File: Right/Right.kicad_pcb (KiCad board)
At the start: 2 copper layers, 106 parts, among them SW1 SW_PUSH, SW10 SW_PUSH, SW100 SW_Push_Dual_R, SW101 SW_Push_Dual_R, SW102 SW_Push_Dual_R, SW11 SW_PUSH, SW12 SW_PUSH, SW13 SW_PUSH, SW14 SW_PUSH, SW15 SW_PUSH, SW16 SW_PUSH, SW17 SW_PUSH, SW18 SW_PUSH, SW19 SW_PUSH, SW2 SW_PUSH, SW20 SW_PUSH, SW200 SW_SPDT, SW21 SW_PUSH, SW22 SW_PUSH, SW23 SW_PUSH, SW24 SW_PUSH, SW25 SW_PUSH, SW26 SW_PUSH, SW27 SW_PUSH, SW28 SW_PUSH, SW29 SW_PUSH, SW3 SW_PUSH, SW30 SW_PUSH, SW31 SW_PUSH, SW32 SW_PUSH, SW33 SW_PUSH, SW34 SW_PUSH, SW35 SW_PUSH, SW36 SW_PUSH, SW37 SW_PUSH, SW38 SW_PUSH, SW39 SW_PUSH, SW4 SW_PUSH, SW40 SW_PUSH, SW41 SW_PUSH, SW42 SW_PUSH, SW43 SW_PUSH, SW44 SW_PUSH, SW45 SW_PUSH, SW5 SW_PUSH, SW6 SW_PUSH, SW7 SW_PUSH, SW8 SW_PUSH, SW9 SW_PUSH, U1 CH25-2032LF, U2 CH25-2032LF

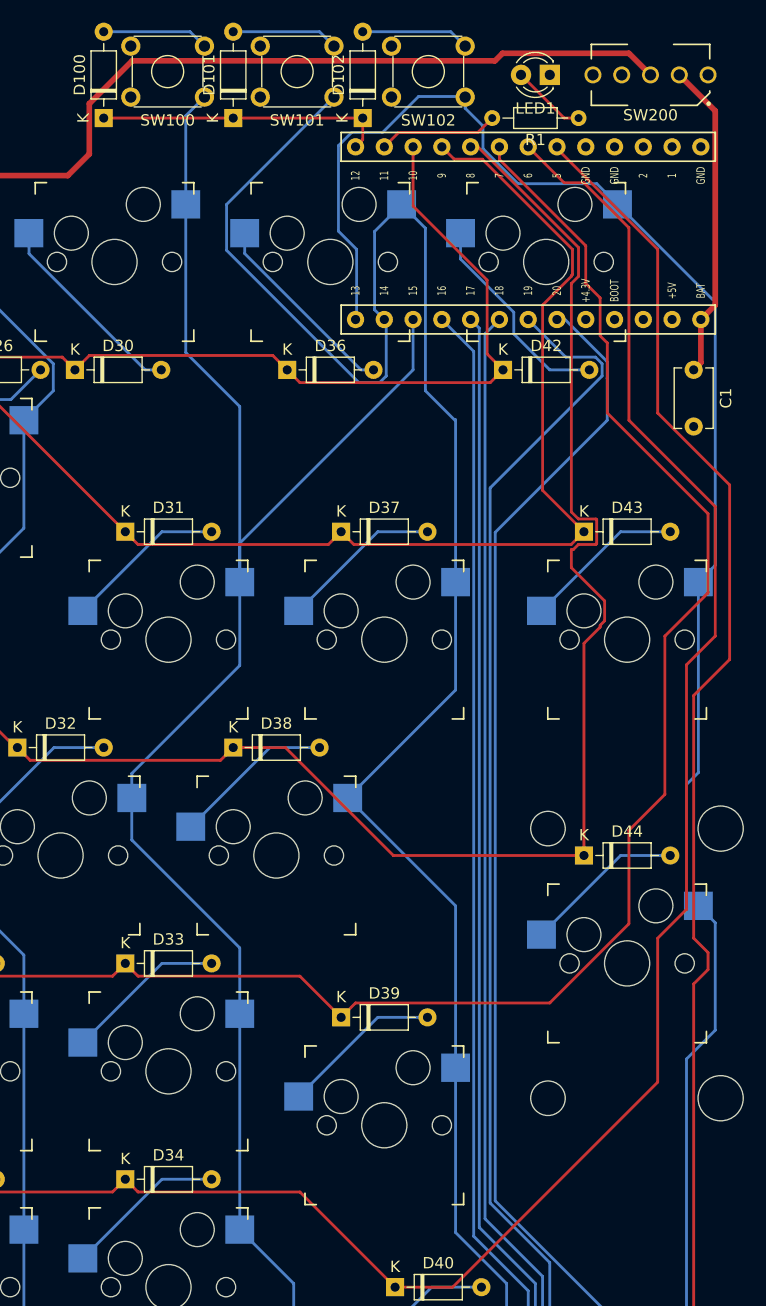
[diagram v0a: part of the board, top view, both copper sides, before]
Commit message: 位置調整
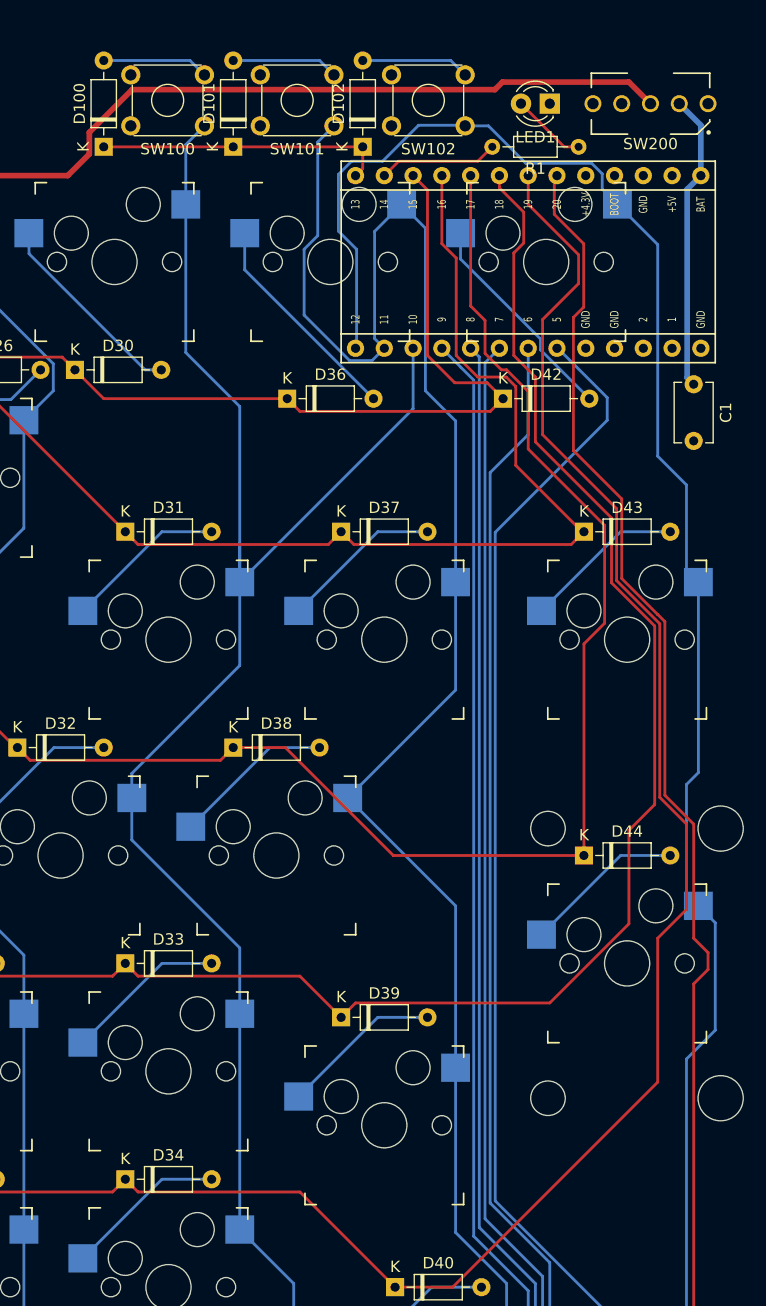
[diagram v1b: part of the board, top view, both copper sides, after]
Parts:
- BPM1: footprint mylibrary:BLEMicroPro_reversed -> mylibrary:BLEMicroPro
- moved BPM1 2.54 mm to (209.6, 59.7)
- moved D100 2.54 mm to (174.6, 49.5)
- moved D101 2.54 mm to (186.1, 49.5)
- moved D102 2.54 mm to (197.5, 49.5)
- moved LED1 2.54 mm to (214.0, 45.7)
- moved R1 2.54 mm to (216.5, 49.5)
- moved SW100 2.54 mm to (183.5, 47.7)
- moved SW101 2.54 mm to (194.9, 47.7)
- moved SW102 2.54 mm to (206.5, 47.7)
- moved SW200 2.54 mm to (222.9, 45.7)
- moved D36 2.54 mm to (190.8, 71.8)
- moved D42 2.54 mm to (209.9, 71.8)
- moved C1 1.27 mm to (226.7, 70.5)
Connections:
- BPM1 pad 10: row1 -> col4
- BPM1 pad 11: row0 -> col5
- BPM1 pad 12: led -> col6
- BPM1 pad 13: rowsys -> col7
- BPM1 pad 14: col7 -> rowsys
- BPM1 pad 15: col6 -> led
- BPM1 pad 16: col5 -> row0
- BPM1 pad 17: col4 -> row1
- BPM1 pad 18: col3 -> row2
- BPM1 pad 19: col2 -> row3
- BPM1 pad 20: col1 -> row4
- BPM1 pad 21: col0 -> row5
- BPM1 pad 6: row5 -> col0
- BPM1 pad 7: row4 -> col1
- BPM1 pad 8: row3 -> col2
- BPM1 pad 9: row2 -> col3
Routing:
- net col6: track 184.5 -> 172.2 mm
- net col1: track 359.0 -> 349.5 mm
- net row2: track 242.3 -> 235.3 mm
- net row3: track 252.9 -> 247.2 mm
- net row1: track 208.2 -> 203.6 mm
- net row5: track 282.5 -> 278.3 mm
- net col7: track 175.4 -> 172.1 mm
- net row4: track 264.6 -> 261.5 mm
- net col0: track 394.1 -> 391.1 mm
- net col2: track 323.9 -> 321.3 mm
- net Net-(D200-Pad1): track 190.7 -> 188.1 mm
- net col4: track 293.6 -> 291.0 mm
- net col3: track 302.4 -> 299.9 mm
- net Net-(D36-Pad2): track 17.4 -> 19.3 mm
- net bat: track 28.1 -> 26.3 mm
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
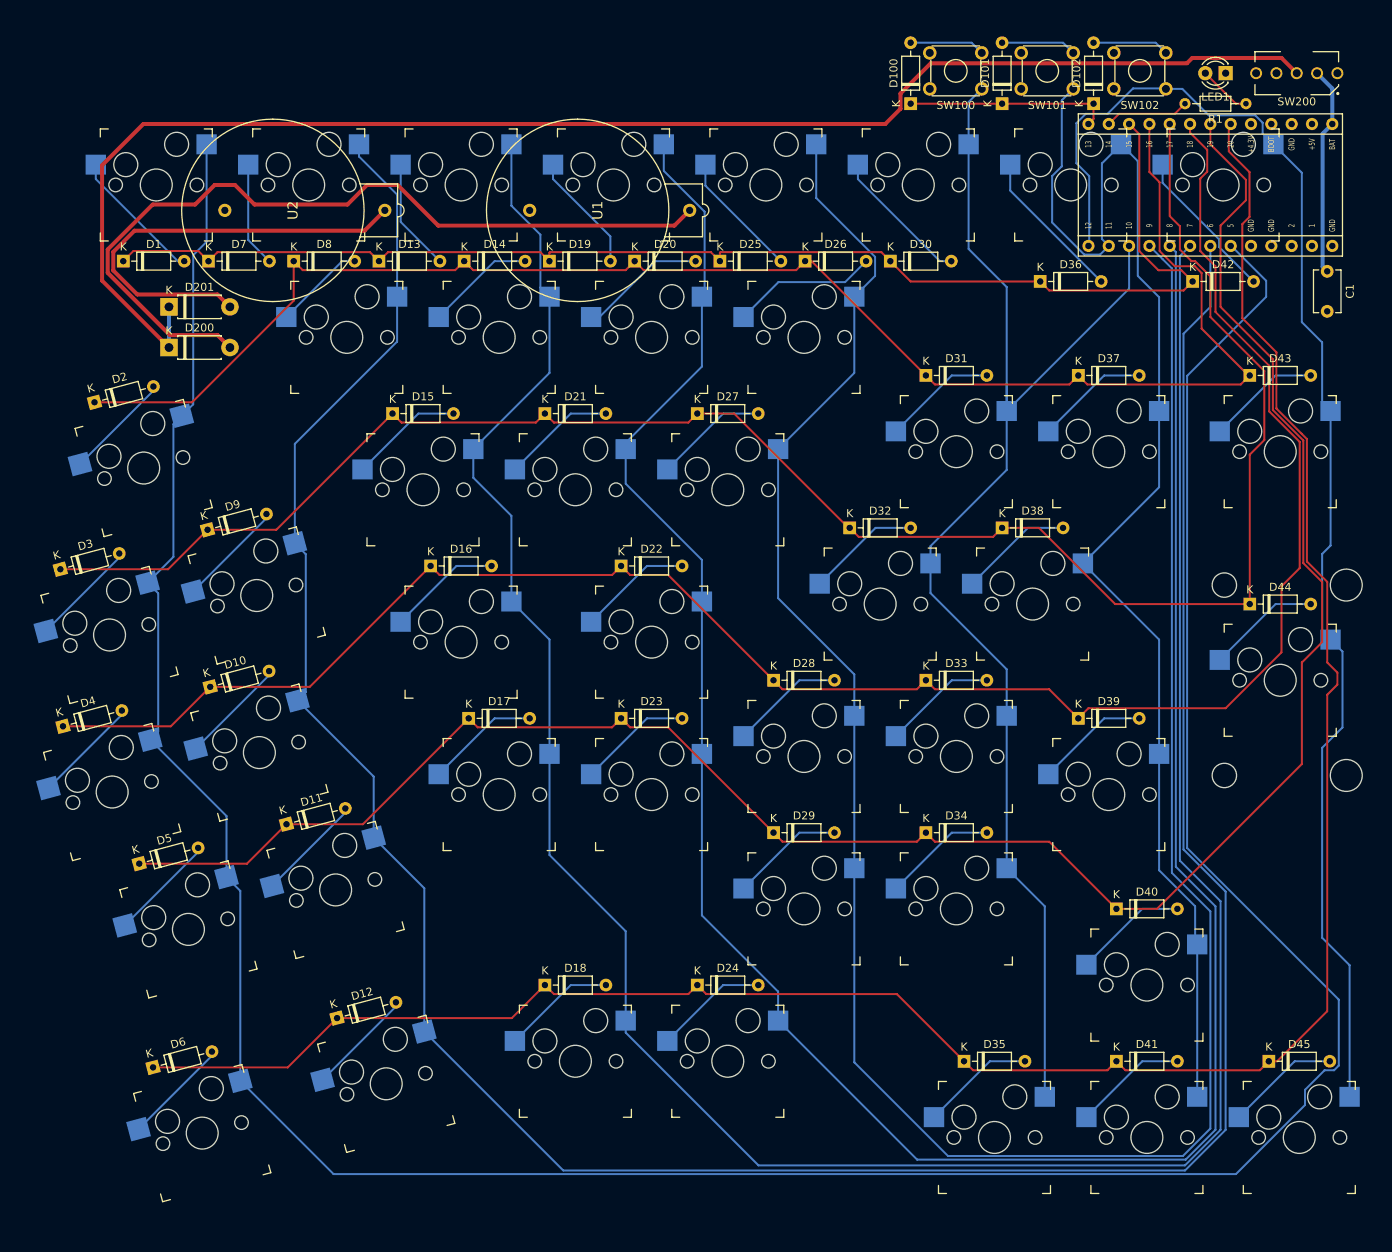
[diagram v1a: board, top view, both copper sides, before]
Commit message: 外枠とスペーサー
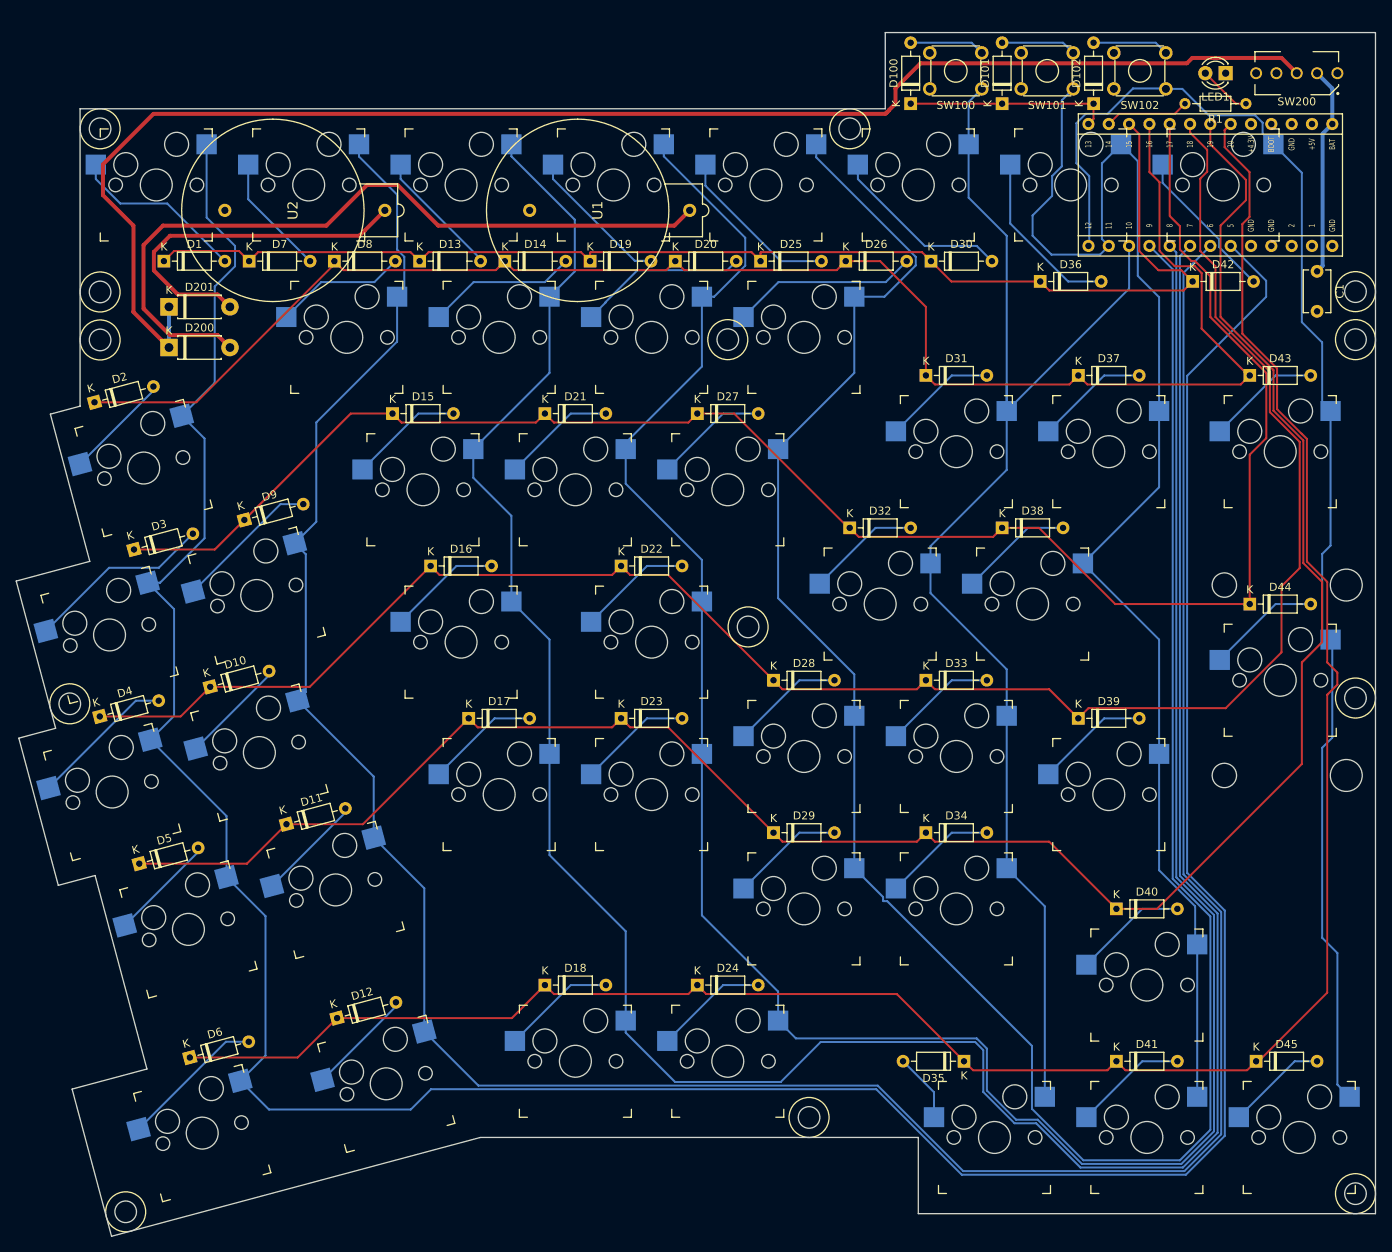
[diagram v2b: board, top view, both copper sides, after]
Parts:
- added REF**: Spacer, mylibrary:Spacer, F.Cu at (151.8, 79.0)
- added REF**: Spacer, mylibrary:Spacer, F.Cu at (73.3, 52.7)
- added REF**: Spacer, mylibrary:Spacer, F.Cu at (73.3, 73.1)
- added REF**: Spacer, mylibrary:Spacer, F.Cu at (76.5, 188.0)
- added REF**: Spacer, mylibrary:Spacer, F.Cu at (230.2, 185.8)
- added REF**: Spacer, mylibrary:Spacer, F.Cu at (230.2, 123.8)
- added REF**: Spacer, mylibrary:Spacer, F.Cu at (69.5, 124.5)
- added REF**: Spacer, mylibrary:Spacer, F.Cu at (161.9, 176.3)
- added REF**: Spacer, mylibrary:Spacer, F.Cu at (167.0, 52.7)
- added REF**: Spacer, mylibrary:Spacer, F.Cu at (154.3, 114.9)
- added REF**: Spacer, mylibrary:Spacer, F.Cu at (73.3, 79.1)
- added REF**: Spacer, mylibrary:Spacer, F.Cu at (230.2, 79.0)
- added REF**: Spacer, mylibrary:Spacer, F.Cu at (230.2, 73.0)
- moved D3 9.53 mm to (77.5, 105.3)
- moved D19 5.08 mm to (134.5, 69.2)
- moved D20 5.08 mm to (145.2, 69.2)
- moved D1 5.08 mm to (81.3, 69.2)
- moved D13 5.08 mm to (113.2, 69.2)
- moved D14 5.08 mm to (123.9, 69.2)
- moved D7 5.08 mm to (91.9, 69.2)
- moved D8 5.08 mm to (102.6, 69.2)
- moved D25 5.08 mm to (155.9, 69.2)
- moved D26 5.08 mm to (166.5, 69.2)
- moved D30 5.08 mm to (177.2, 69.2)
- moved D6 4.76 mm to (84.5, 168.8)
- moved D4 4.76 mm to (73.3, 126.1)
- moved D9 4.76 mm to (91.3, 101.6)
- moved D45 1.59 mm to (217.8, 169.2)
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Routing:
- net Net-(D201-Pad2): track 54.9 -> 44.7 mm
- net row2: track 235.3 -> 225.3 mm
- net Net-(D3-Pad2): track 13.5 -> 23.4 mm
- net col2: track 321.3 -> 331.1 mm
- net col3: track 299.9 -> 308.4 mm
- net Net-(D200-Pad2): track 103.1 -> 95.0 mm
- net Net-(D20-Pad2): track 16.0 -> 22.1 mm
- net row5: track 278.3 -> 272.2 mm
- net Net-(D1-Pad2): track 17.1 -> 23.0 mm
- net Net-(D35-Pad2): track 14.3 -> 8.59 mm
- net row3: track 247.2 -> 242.1 mm
- net row0: track 166.3 -> 161.2 mm
- net Net-(D25-Pad2): track 16.0 -> 21.1 mm
- net Net-(D14-Pad2): track 13.7 -> 18.8 mm
- net Net-(D8-Pad2): track 11.4 -> 16.5 mm
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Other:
- board outline added: 169.9 x 150.5 mm
